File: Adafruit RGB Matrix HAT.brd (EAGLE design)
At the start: 65 x 56.5 mm, 42 parts, among them IC3 MAX4866T, Q1 AOD514, Q2 AOD417, U1 CAT24C32, U2 2.1MMJACKSMT, U3 74AHCT245, U4 DS1307, U5 74AHCT245, Y1 32.768kHz

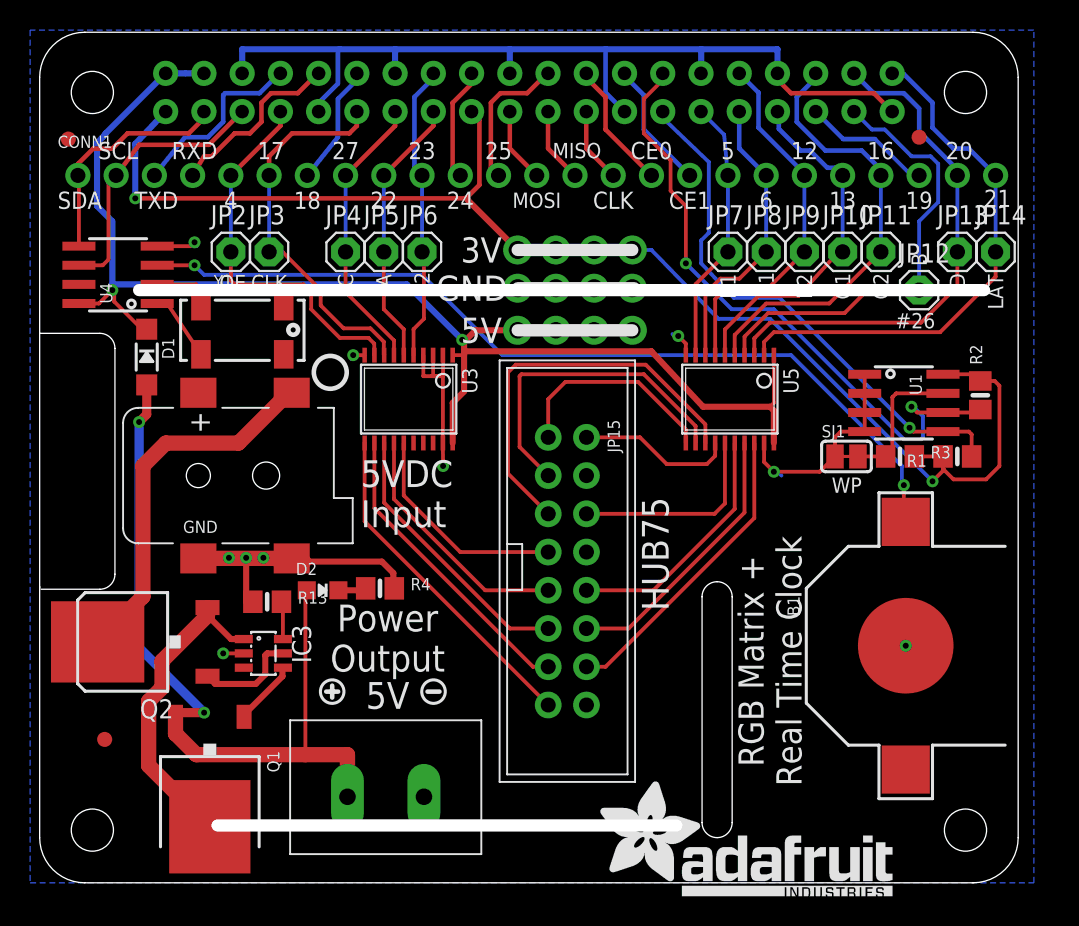
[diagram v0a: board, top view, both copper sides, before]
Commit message: Update to Rev C
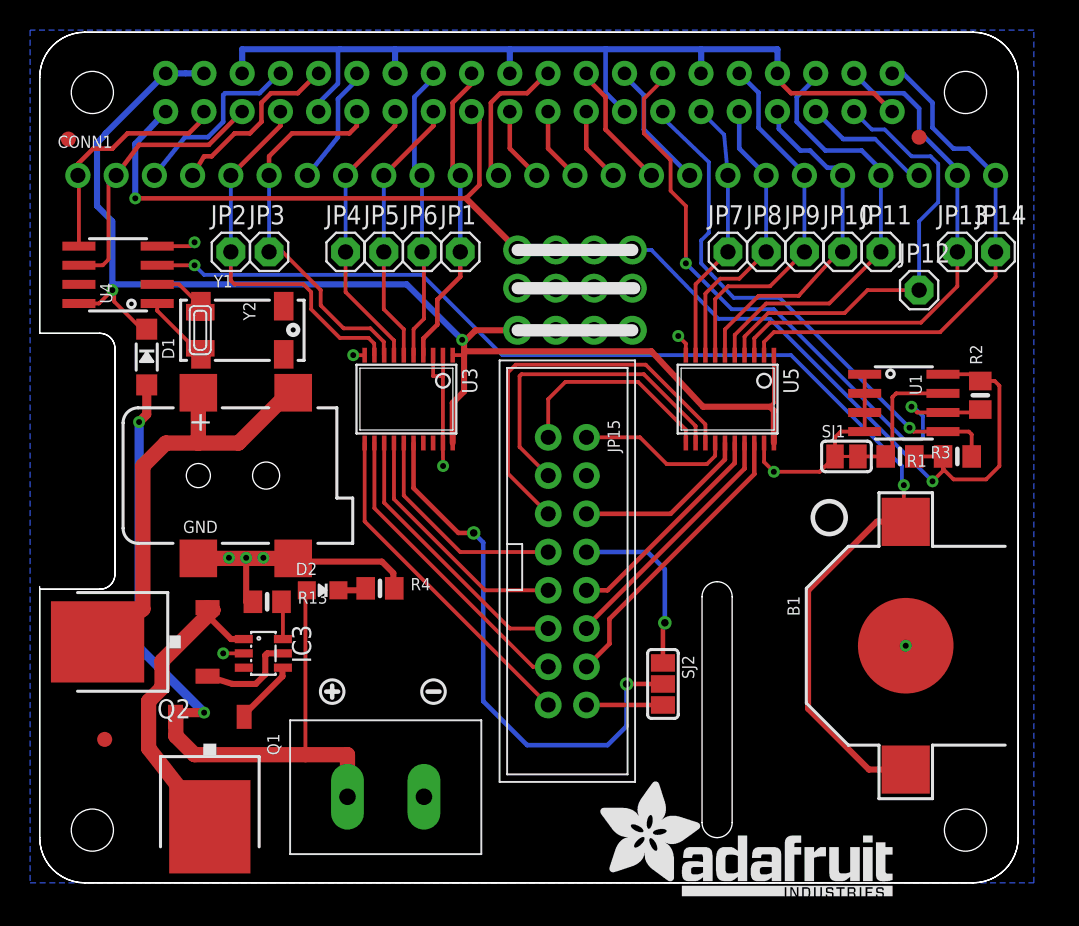
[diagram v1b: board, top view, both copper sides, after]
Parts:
- removed U2: 2.1MMJACKSMT, adafruit:DCJACK_2MM_SMT
- added JP1: (no value), pinhead-ez:1X01
- added PLABEL0: (no value), pinguin:PLABEL0
- added PLABEL1: (no value), pinguin:PLABEL1
- added PLABEL10: (no value), pinguin:PLABEL10
- added PLABEL11: (no value), pinguin:PLABEL11
- added PLABEL12: (no value), pinguin:PLABEL12
- added PLABEL13: (no value), pinguin:PLABEL13
- added PLABEL14: (no value), pinguin:PLABEL14
- added PLABEL15: (no value), pinguin:PLABEL15
- added PLABEL16: (no value), pinguin:PLABEL16
- added PLABEL17: (no value), pinguin:PLABEL17
- added PLABEL18: (no value), pinguin:PLABEL18
- added PLABEL19: (no value), pinguin:PLABEL19
- added PLABEL2: (no value), pinguin:PLABEL2
- added PLABEL20: (no value), pinguin:PLABEL20
- added PLABEL21: (no value), pinguin:PLABEL21
- added PLABEL22: (no value), pinguin:PLABEL22
- added PLABEL23: (no value), pinguin:PLABEL23
- added PLABEL24: (no value), pinguin:PLABEL24
- added PLABEL25: (no value), pinguin:PLABEL25
- added PLABEL26: (no value), pinguin:PLABEL26
- added PLABEL27: (no value), pinguin:PLABEL27
- added PLABEL28: (no value), pinguin:PLABEL28
- added PLABEL29: (no value), pinguin:PLABEL29
- added PLABEL3: (no value), pinguin:PLABEL3
- added PLABEL30: (no value), pinguin:PLABEL30
- added PLABEL31: (no value), pinguin:PLABEL31
- added PLABEL32: (no value), pinguin:PLABEL32
- added PLABEL33: (no value), pinguin:PLABEL33
- added PLABEL34: (no value), pinguin:PLABEL34
- added PLABEL35: (no value), pinguin:PLABEL35
- added PLABEL36: (no value), pinguin:PLABEL36
- added PLABEL37: (no value), pinguin:PLABEL37
- added PLABEL38: (no value), pinguin:PLABEL38
- added PLABEL39: (no value), pinguin:PLABEL39
- added PLABEL4: (no value), pinguin:PLABEL4
- added PLABEL40: (no value), pinguin:PLABEL40
- added PLABEL41: (no value), pinguin:PLABEL41
- added PLABEL42: (no value), pinguin:PLABEL42
- added PLABEL43: (no value), pinguin:PLABEL43
- added PLABEL44: (no value), pinguin:PLABEL44
- added PLABEL45: (no value), pinguin:PLABEL45
- added PLABEL46: (no value), pinguin:PLABEL46
- added PLABEL47: (no value), pinguin:PLABEL47
- added PLABEL48: (no value), pinguin:PLABEL48
- added PLABEL49: (no value), pinguin:PLABEL49
- added PLABEL5: (no value), pinguin:PLABEL5
- added PLABEL50: (no value), pinguin:PLABEL50
- added PLABEL51: (no value), pinguin:PLABEL51
- added PLABEL6: (no value), pinguin:PLABEL6
- added PLABEL7: (no value), pinguin:PLABEL7
- added PLABEL8: (no value), pinguin:PLABEL8
- added PLABEL9: (no value), pinguin:PLABEL9
- added SJ2: (no value), microbuilder:SOLDERJUMPER_2WAY_OPEN_NOPASTE
- added X1: 2.1mm DC, adafruit_electromech:DCJACK_2MM_SMT
- added Y2: 32.768kHz, microbuilder:XTAL3215
- FID1, FID2, FID3: value FIDUCIAL"" -> FIDUCIAL_1MM
- Q2: device transistor-power:D-PAK_TO252AA -> microbuilder:TO252
- RPI1: device microbuilder:PI_HAT_SLOTS -> adafruit_sbc:PI_HAT_SLOTS
- moved U$3 34.5 mm to (52.5, 24.3), turned to 90 degrees
- moved Q2 1.14 mm to (7.49, 16.0)
- moved Q1 1.14 mm to (11.3, 7.37)
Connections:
- new net M1_E: SJ2.2, U3.16
- new net M1_E': JP15.8, SJ2.1
- new net M1_E'': JP15.16, SJ2.3
- net 5VIN: now also Q2.3, X1.1, X1.1'; no longer Q2.4, U2.PWR2
- net GND: now also X1.2, X1.3; no longer JP15.16, JP15.8, U2.GND, U2.GNDBREAK, U3.4
- net GPIO24: now also JP1.1, U3.4
- net N$14: now also B1.+$2
- net N$2: now also Y2.P$1
- net N$3: now also Y2.P$2
- net N$5: now also Q2.2; no longer Q2.3
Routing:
- net M1_E: track 0.00 -> 36.1 mm, vias 0 -> 2
- net N$14: track 58.8 -> 83.2 mm
- net GPIO24: track 7.51 -> 20.5 mm
- net M1_E': track 0.00 -> 11.9 mm, vias 0 -> 1
- net GND: track 127.9 -> 119.7 mm
- net M1_E'': track 0.00 -> 5.08 mm
- net 5VIN: track 24.8 -> 28.6 mm
- net M1_B: track 16.5 -> 14.7 mm
- net M1_G2: track 13.5 -> 11.8 mm
- net M1_D: track 18.3 -> 16.7 mm
- net LAT: track 20.2 -> 19.5 mm
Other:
- outline, holes or cut-outs redrawn
- board text added: "8"
- board text added: "E"
